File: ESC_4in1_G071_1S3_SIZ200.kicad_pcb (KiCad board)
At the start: 4 copper layers, 27 x 28 mm, 176 parts, among them J1 Conn_01x10, U1 STM32G071GBU6, U10 NCP81161MNTBG, U11 SIZ200DT-T1-GE3, U12 NCP81161MNTBG, U13 SIZ200DT-T1-GE3, U14 TPS630701, U15 TPS72733DSE, U16 INA186A2, U17 STM32G071GBU6, U18 NCP81161MNTBG, U19 SIZ200DT-T1-GE3, U2 NCP81161MNTBG, U20 NCP81161MNTBG, U21 STM32G071GBU6, U22 SIZ200DT-T1-GE3, U23 NCP81161MNTBG, U24 SIZ200DT-T1-GE3, U25 NCP81161MNTBG, U26 SIZ200DT-T1-GE3, U27 NCP81161MNTBG, U28 STM32G071GBU6, U29 SIZ200DT-T1-GE3, U3 SIZ200DT-T1-GE3, U30 NCP81161MNTBG, U31 SIZ200DT-T1-GE3, U4 NCP81161MNTBG, U5 SIZ200DT-T1-GE3, U6 NCP81161MNTBG, U7 SIZ200DT-T1-GE3, U8 NCP81161MNTBG, U9 SIZ200DT-T1-GE3

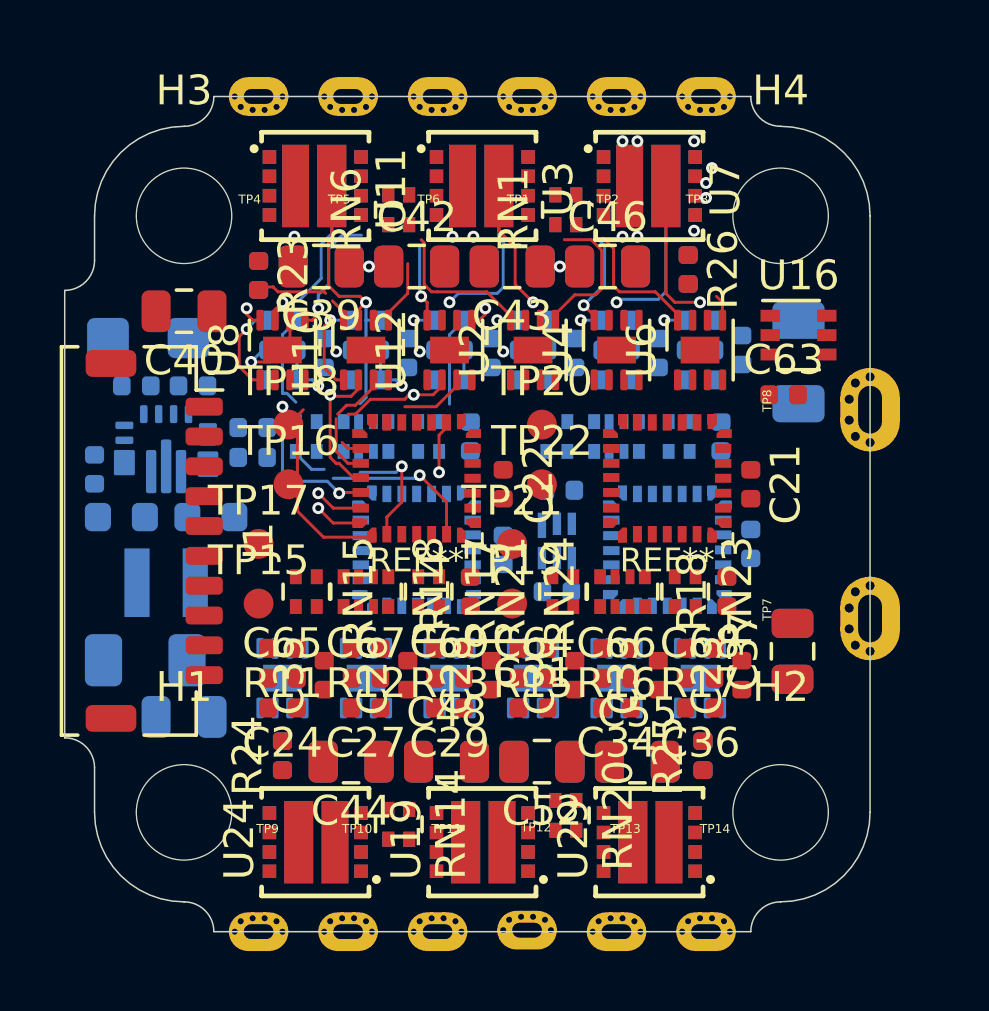
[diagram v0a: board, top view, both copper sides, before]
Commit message: update design files
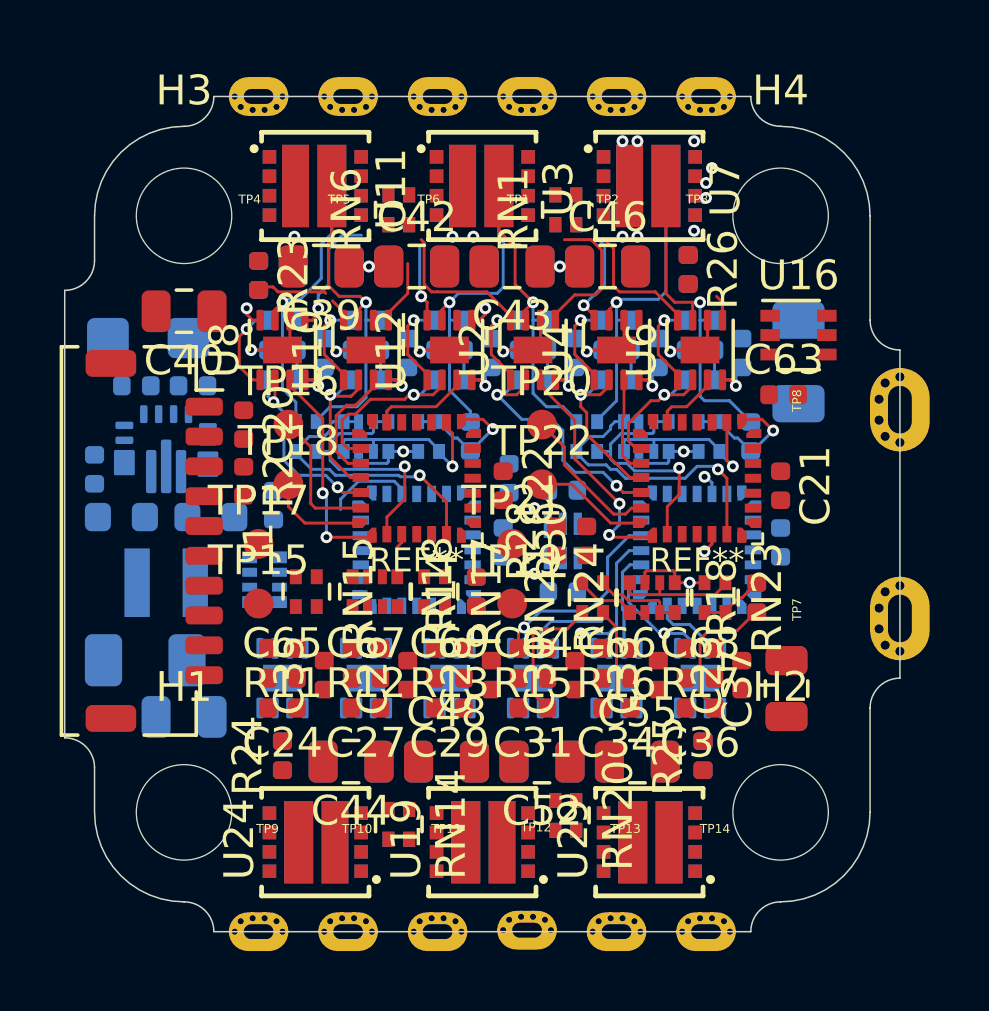
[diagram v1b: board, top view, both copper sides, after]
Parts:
- added R27: 1k, Resistor_SMD:R_0402_1005Metric, B.Cu at (129.0, 74.7)
- added R28: 1k, Resistor_SMD:R_0402_1005Metric, F.Cu at (138.5, 75.9)
- added R29: 1k, Resistor_SMD:R_0402_1005Metric, B.Cu at (136.9, 73.8)
- added R30: 1k, Resistor_SMD:R_0402_1005Metric, F.Cu at (139.5, 75.9)
- added RN2: 1k, 11_PSoC_FC_whoop:R_Array_Convex_4x0402_dense, B.Cu at (128.7, 77.2)
- C20, R2: moved to F.Cu
- moved TP16 2.00 mm to (129.5, 72.0)
- moved TP18 2.00 mm to (129.5, 74.0)
- moved C37 1.27 mm to (146.2, 80.8)
- moved C50 1.27 mm to (146.2, 80.8)
- moved R18 1.02 mm to (145.2, 77.8)
- moved RN21 1.02 mm to (139.7, 77.8)
- moved RN23 1.02 mm to (143.8, 77.8)
- moved RN24 1.02 mm to (141.7, 77.8)
- moved C21 1.00 mm to (146.0, 74.0)
- moved C32 1.00 mm to (146.0, 76.0)
- moved R6 1.00 mm to (145.0, 72.4)
- moved RN7 1.00 mm to (143.6, 72.4)
- moved RN8 1.00 mm to (139.5, 72.4)
- moved RN9 1.00 mm to (141.5, 72.4)
- moved TP7 1.00 mm to (150.0, 78.5)
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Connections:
- J1 pad 5: /ESC1_IN -> Net-(J1-Pad5)
- J1 pad 6: /ESC2_IN -> Net-(J1-Pad6)
- J1 pad 7: /ESC3_IN -> Net-(J1-Pad7)
- J1 pad 8: /ESC4_IN -> Net-(J1-Pad8)
- RN24 pad 5: /ESC3_Y -> GND
- RN24 pad 6: GND -> /ESC3_Y
- RN24 pad 7: /ESC3_Y -> GND
- RN24 pad 8: GND -> /ESC3_Y
- RN9 pad 5: /ESC1_Y -> GND
- RN9 pad 6: GND -> /ESC1_Y
- RN9 pad 7: /ESC1_Y -> GND
- RN9 pad 8: GND -> /ESC1_Y
- U1 pad 26: /ESCx_tele -> Net-(R30-Pad2)
- U17 pad 26: /ESCx_tele -> Net-(R28-Pad2)
- U21 pad 26: /ESCx_tele -> Net-(R27-Pad2)
- U28 pad 26: /ESCx_tele -> Net-(R29-Pad2)
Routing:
- net GND: track 3.05 -> 25.0 mm, vias 10 -> 15
- net +5V: track 4.60 -> 17.7 mm, vias 2 -> 6
- net /ESC1_MA: track 0.00 -> 10.3 mm, vias 0 -> 1
- net /ESC1_A_PWM: track 0.00 -> 8.96 mm, vias 0 -> 2
- net /ESC1_MB: track 0.00 -> 8.31 mm, vias 0 -> 1
- net /ESC1_A_EN: track 0.00 -> 7.92 mm, vias 0 -> 2
- net /ESC3_A_PWM: track 0.00 -> 7.37 mm, vias 0 -> 1
- net /ESC1_Y: track 0.00 -> 6.41 mm, vias 0 -> 1
- net /ESC1_C: track 4.87 -> 11.2 mm
- net /ESC1_A: track 4.37 -> 10.5 mm
- net /ESC1_B_PWM: track 0.00 -> 6.03 mm, vias 0 -> 1
- net /ESC1_B: track 5.35 -> 10.8 mm
- net /ESC1_SWDIO: track 0.00 -> 5.00 mm
- net /ESC1_C_PWM: track 0.00 -> 4.92 mm, vias 0 -> 1
- net /ESC3_B_PWM: track 0.00 -> 4.90 mm, vias 0 -> 1
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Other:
- board size 27 x 28 mm -> 28 x 28 mm
